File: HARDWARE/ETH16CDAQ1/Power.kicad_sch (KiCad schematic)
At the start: 32 parts, among them J501 1715721, Q501 SI5618A, Q502 MMBT3904, U501 PDME2-S24-D24-S, U502 PDME2-S24-S9-S, U503 TLE4476DXT, U504 TPS7A39

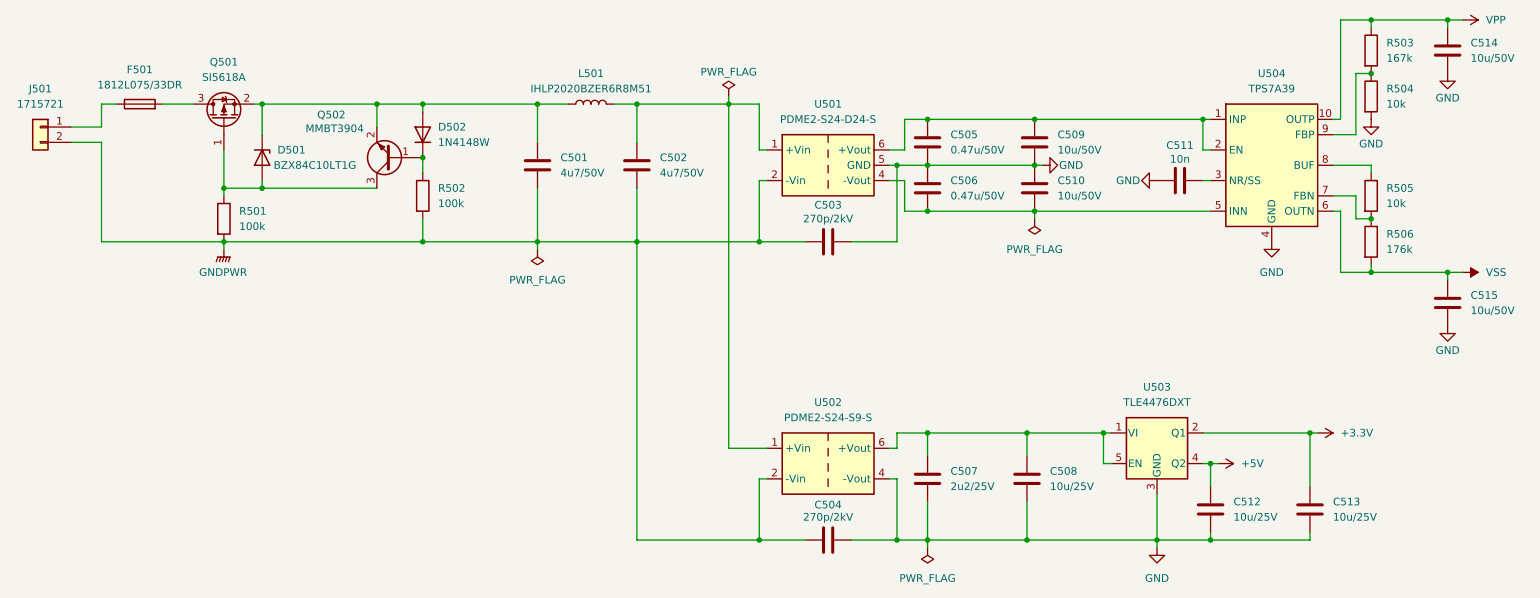
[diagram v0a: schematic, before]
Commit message: Development
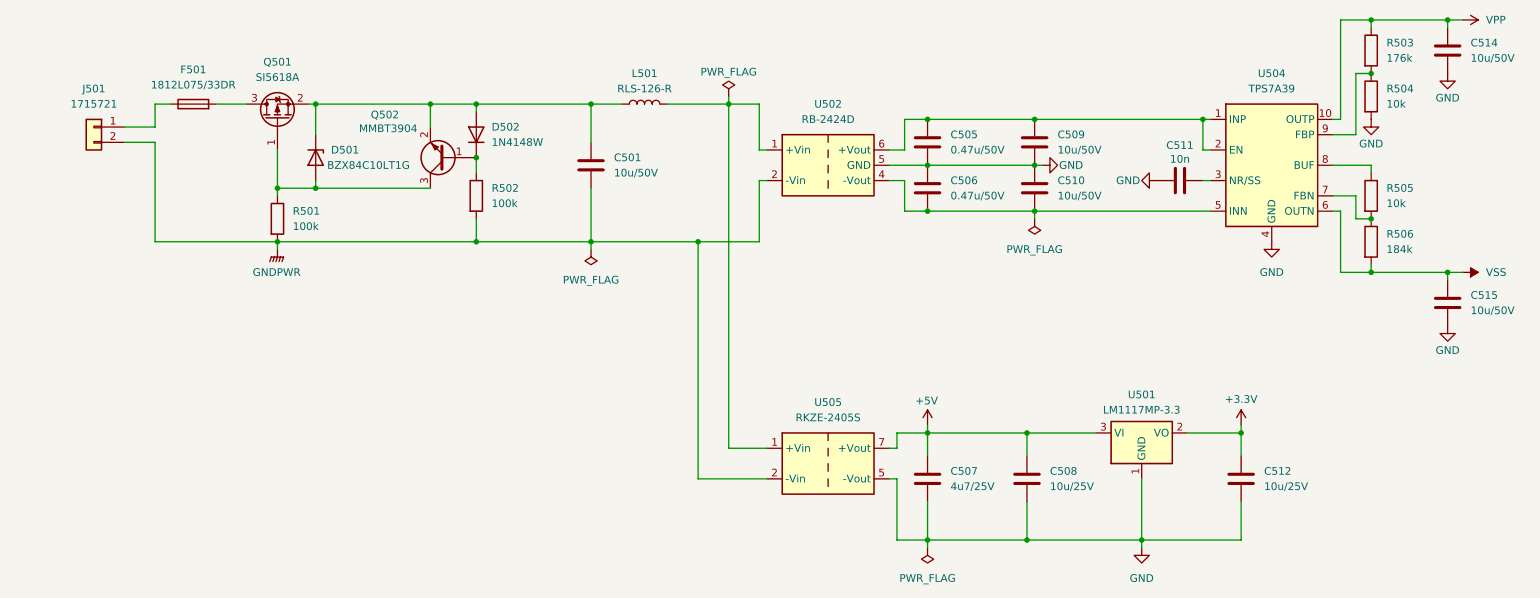
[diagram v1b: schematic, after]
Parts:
- removed C502: 4u7/50V, Capacitor_SMD:C_1206_3216Metric_Pad1.33x1.80mm_HandSolder, symbol Device:C
- removed C503, C504: 270p/2kV, Capacitor_SMD:C_1206_3216Metric_Pad1.33x1.80mm_HandSolder, symbol Device:C
- removed C513: 10u/25V, Capacitor_SMD:C_1206_3216Metric_Pad1.33x1.80mm_HandSolder, symbol Device:C
- removed U501: PDME2-S24-D24-S, ETH16CDAQ1:CONV_PDME2-S24-D24-S, symbol ETH16CDAQ1:PDME2-S24-D24-S
- removed U502: PDME2-S24-S9-S, ETH16CDAQ1:CONV_PDME2-S24-S9-S, symbol ETH16CDAQ1:PDME2-S24-S9-S
- removed U503: TLE4476DXT, Package_TO_SOT_SMD:TO-252-4, symbol ETH16CDAQ1:TLE4476D
- added U501: LM1117MP-3.3, Package_TO_SOT_SMD:SOT-223-3_TabPin2, symbol Regulator_Linear:LM1117MP-3.3
- added U502: RB-2424D, ETH16CDAQ1:CONV_RB-2424D, symbol ETH16CDAQ1:RB-2424D
- added U505: RKZE-2405S, ETH16CDAQ1:CONV_RKZE-2405S, symbol ETH16CDAQ1:RKZE-2405S
- C501: value 4u7/50V -> 10u/50V
- C507: value 2u2/25V -> 4u7/25V
- L501: value IHLP2020BZER6R8M51 -> RLS-126-R; footprint Inductor_SMD:L_Vishay_IHLP-2020 -> ETH16CDAQ1:IND_RLS-126-R
- R503: value 167k -> 176k
- R506: value 176k -> 184k
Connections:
- net +3.3V: now also C512.1, U501.2 (VO)
- net +5V: now also C507.1, C508.1, U501.3 (VI), U505.7 (+Vout); no longer C512.1
- net GND: now also U501.1 (GND), U502.5 (GND), U505.5 (-Vout)
- net GNDPWR: now also U502.2 (-Vin), U505.2 (-Vin)
- net at L501.2: now also U502.1 (+Vin), U505.1 (+Vin)
- net at C506.2, C510.2, U504.5 (INN): now also U502.4 (-Vout)
- net at C505.1, C509.1, U504.1 (INP)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: now also U502.6 (+Vout)
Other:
- moved on the sheet: C501, C512, D501, D502, F501, J501, L501, Q501, Q502, R501, R502
